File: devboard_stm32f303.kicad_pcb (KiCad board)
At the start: 2 copper layers, 50 x 17.8 mm, 23 parts, among them J1 Conn_01x04, J2 USB_B_Mini, J3 Conn_01x20, J4 Conn_01x20, SW1 SW_Push, U1 STM32F303CCTx, U2 AMS1117-3.3, Y1 Crystal_Small

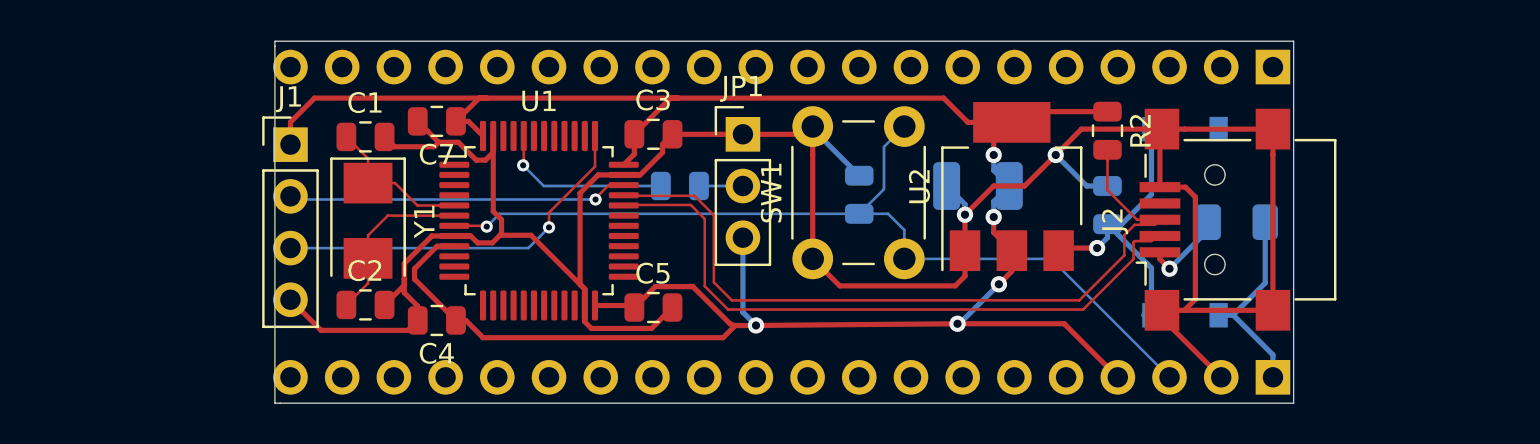
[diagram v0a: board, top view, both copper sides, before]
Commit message: Start new routing
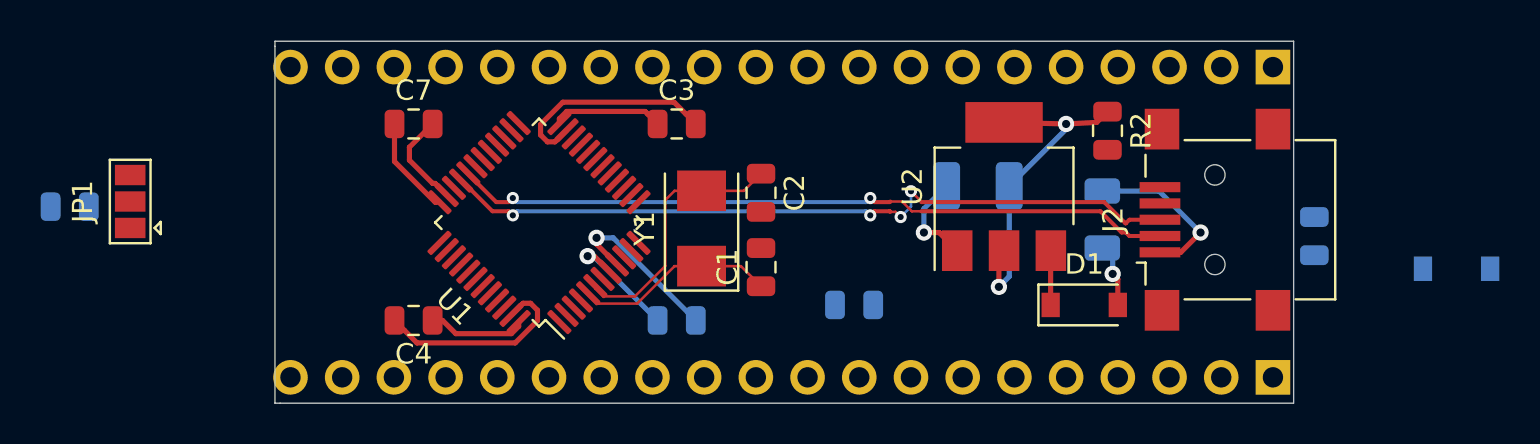
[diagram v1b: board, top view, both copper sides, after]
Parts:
- removed J1: Conn_01x04, Connector_PinHeader_2.54mm:PinHeader_1x04_P2.54mm_Vertical
- removed SW1: SW_Push, Button_Switch_THT:SW_PUSH_6mm
- C5: moved to B.Cu
- D1: moved to F.Cu
- JP1: footprint Connector_PinHeader_2.54mm:PinHeader_1x03_P2.54mm_Vertical -> Jumper:SolderJumper-3_P1.3mm_Open_Pad1.0x1.5mm
- moved JP1 30.3 mm to (84.6, 30.2), turned to 90 degrees
- moved R1 30.0 mm to (81.6, 30.5)
- moved C1 20.5 mm to (115.6, 33.4), turned to 90 degrees
- moved C2 20.2 mm to (115.6, 29.8), turned to 270 degrees
- moved Y1 16.4 mm to (112.6, 31.6), turned to 90 degrees
- moved D2 15.0 mm to (149.7, 33.5)
- moved C8 10.3 mm to (142.7, 31.9)
- moved F1 6.61 mm to (132.3, 31.1), turned to 270 degrees
- moved C6 5.42 mm to (120.1, 35.3), turned to 0 degrees
- moved D1 4.98 mm to (131.4, 35.3)
- moved C5 1.31 mm to (111.4, 36.1), turned to 180 degrees
- moved C3 1.25 mm to (111.4, 26.4)
- moved C7 1.15 mm to (98.5, 26.4), turned to 0 degrees
- moved C4 1.14 mm to (98.5, 36.1)
- moved U2 0.38 mm to (127.5, 29.5)
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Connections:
- net Net-(J3-Pad18) renamed PA15
- J3 pad 1: Net-(J3-Pad1) -> PA9
- J3 pad 10: Net-(J3-Pad10) -> PB2
- J3 pad 11: Net-(J3-Pad11) -> PB1
- J3 pad 12: Net-(J3-Pad12) -> PB0
- J3 pad 13: Net-(J3-Pad13) -> PA4
- J3 pad 14: Net-(J3-Pad14) -> PA5
- J3 pad 15: Net-(J3-Pad15) -> PA6
- J3 pad 16: Net-(J3-Pad16) -> PA7
- J3 pad 17: Net-(J3-Pad17) -> PA8
- J3 pad 2: Net-(J3-Pad2) -> PA10
- J3 pad 3: Net-(J3-Pad3) -> GND
- J3 pad 4: Net-(J3-Pad4) -> GND
- J3 pad 5: Net-(J3-Pad5) -> PB7
- J3 pad 6: Net-(J3-Pad6) -> PB6
- J3 pad 7: Net-(J3-Pad7) -> PB5
- J3 pad 8: Net-(J3-Pad8) -> PB4
- J3 pad 9: Net-(J3-Pad9) -> PB3
- J4 pad 10: Net-(J4-Pad10) -> PB14
- J4 pad 11: Net-(J4-Pad11) -> PB15
- J4 pad 12: Net-(J4-Pad12) -> PB9
- J4 pad 13: Net-(J4-Pad13) -> PB10
- J4 pad 14: Net-(J4-Pad14) -> PB11
- J4 pad 15: Net-(J4-Pad15) -> PB12
- J4 pad 16: Net-(J4-Pad16) -> SWCLK
- J4 pad 17: Net-(J4-Pad17) -> SWDIO
- J4 pad 18: Net-(J4-Pad18) -> RESET
- J4 pad 5: Net-(J4-Pad5) -> PA2
- J4 pad 6: Net-(J4-Pad6) -> PA1
- J4 pad 7: Net-(J4-Pad7) -> PA0
- J4 pad 8: Net-(J4-Pad8) -> PB8
- J4 pad 9: Net-(J4-Pad9) -> PB13
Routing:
- net GND: track 133.3 -> 36.5 mm
- net +3V3: track 117.4 -> 40.0 mm, vias 5 -> 3
- net RESET: track 44.8 -> 0.00 mm, vias 1 -> 0
- net SWCLK: track 18.5 -> 0.00 mm, vias 1 -> 0
- net SWDIO: track 16.8 -> 0.00 mm, vias 1 -> 0
- net Net-(C8-Pad1): track 15.1 -> 2.67 mm, vias 1 -> 0
- net BOOT0: track 8.63 -> 0.00 mm, vias 1 -> 0
- net VBUS: track 9.93 -> 3.11 mm, vias 0 -> 1
- net OSC_OUT: track 8.49 -> 12.8 mm
- net Net-(F1-Pad1): track 4.16 -> 8.07 mm
- net D-: track 32.4 -> 35.6 mm, vias 0 -> 2
- net OSC_IN: track 7.40 -> 9.87 mm
- net Net-(JP1-Pad2): track 2.16 -> 0.00 mm
- net D+: track 37.8 -> 37.1 mm, vias 0 -> 4
